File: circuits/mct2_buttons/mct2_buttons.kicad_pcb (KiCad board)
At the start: 2 copper layers, 62.5 x 28 mm, 35 parts, among them J1 Conn_01x08, SW1 B3F-1052, SW10 B3F-1052, SW11 B3F-1052, SW12 B3F-1052, SW13 OS102011MS2QN1C, SW14 OS102011MS2QN1C, SW2 B3F-1052, SW3 B3F-1052, SW4 B3F-1052, SW5 B3F-1052, SW6 B3F-1052, SW7 B3F-1052, SW8 B3F-1052, SW9 B3F-1052, U1 TCA8418

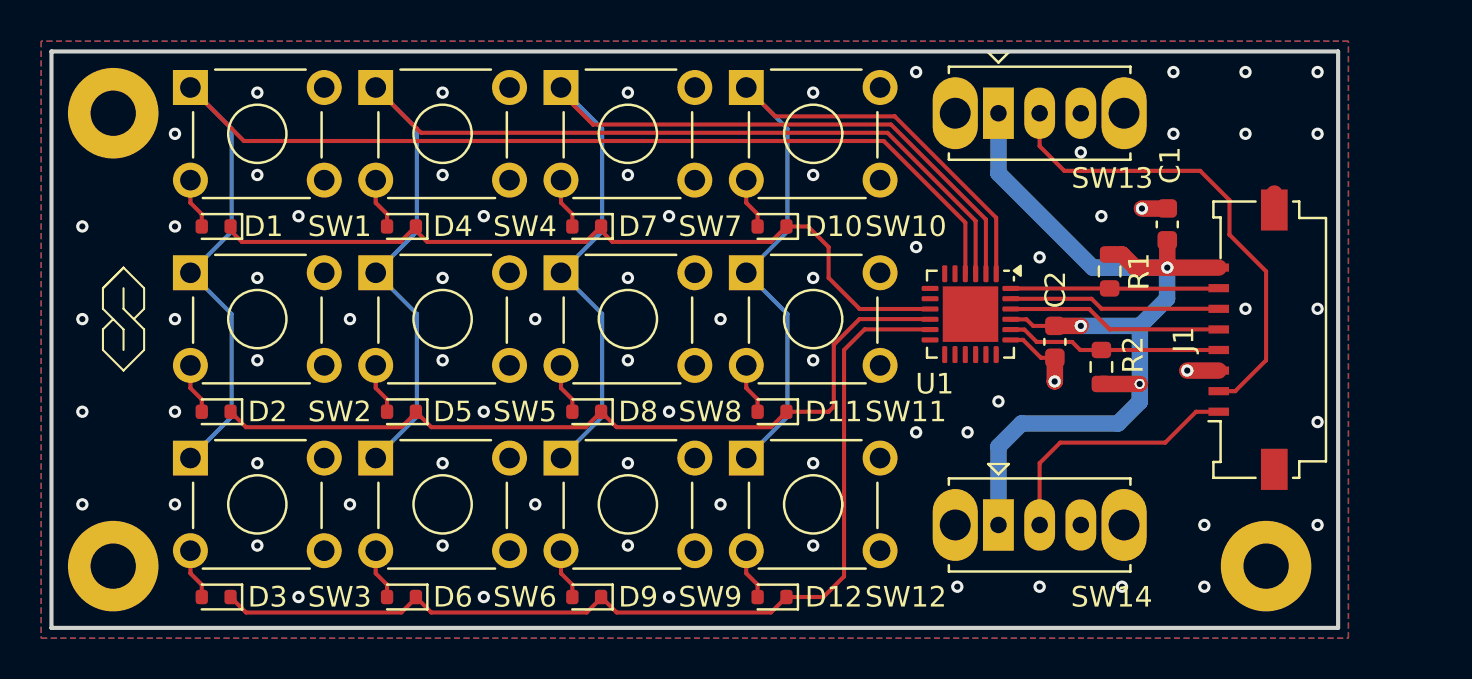
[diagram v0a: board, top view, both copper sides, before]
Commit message: Aug 3, 2024
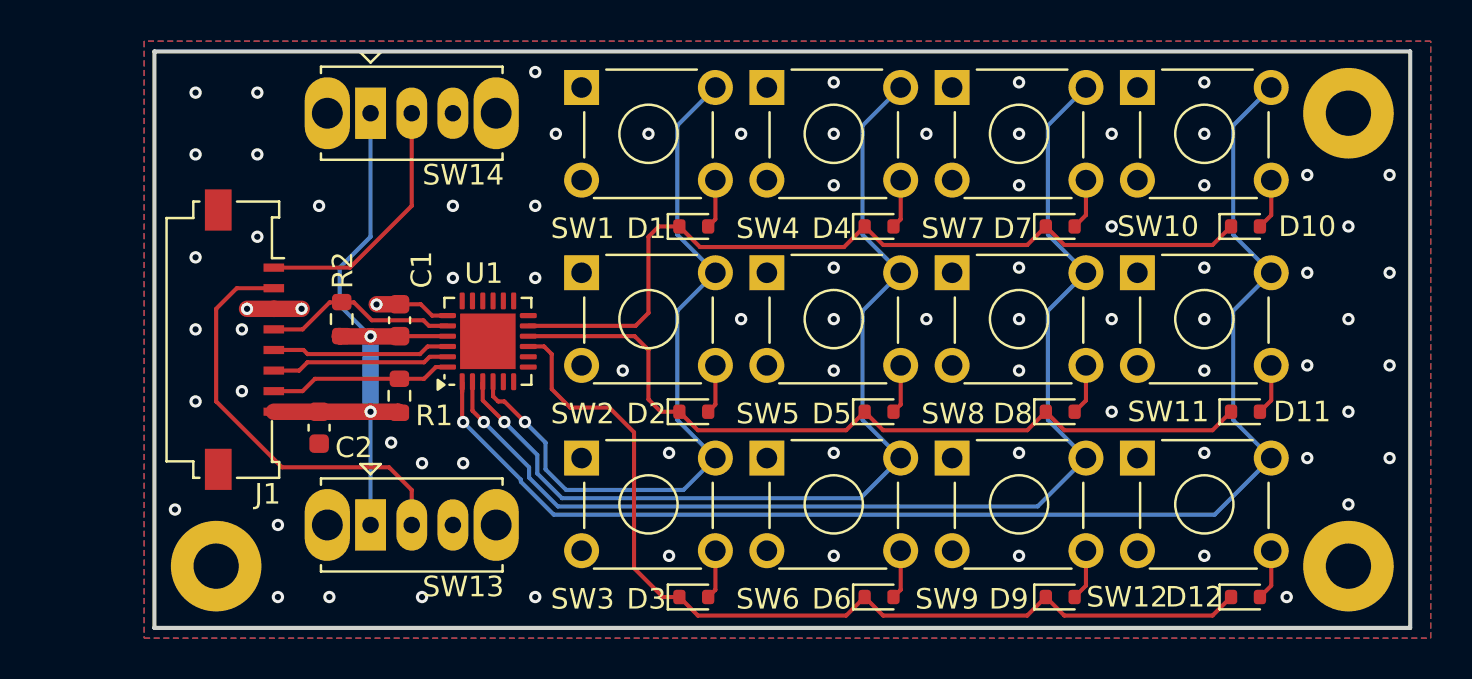
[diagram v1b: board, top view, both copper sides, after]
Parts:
- removed H4: MountingHole, MountingHole:MountingHole_2.2mm_M2_Pad
- added H3: MountingHole, MountingHole:MountingHole_2.2mm_M2_Pad, F.Cu at (98.0, 65.0)
- moved H2 63.9 mm to (98.0, 43.0)
- moved J1 47.7 mm to (44.9, 54.0), turned to -90 degrees
- moved C1 37.6 mm to (51.9, 53.1)
- moved R2 37.0 mm to (49.1, 53.0)
- moved SW13 36.5 mm to (52.5, 63.0)
- moved SW14 36.5 mm to (52.5, 43.0)
- moved C2 36.0 mm to (48.0, 58.3)
- moved R1 35.0 mm to (51.9, 56.7), turned to 90 degrees
- moved U1 23.5 mm to (56.2, 54.1), turned to 90 degrees
- moved D1 23.2 mm to (66.2, 48.5), turned to 0 degrees
- moved D2 23.2 mm to (66.2, 57.5), turned to 0 degrees
- moved D3 23.2 mm to (66.2, 66.5), turned to 0 degrees
- moved D4 23.2 mm to (75.2, 48.5), turned to 0 degrees
- moved D5 23.2 mm to (75.2, 57.5), turned to 0 degrees
- moved D6 23.2 mm to (75.2, 66.5), turned to 0 degrees
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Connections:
- net Net-(D11-K) renamed COL1
- D1 pad 1: Net-(D1-K) -> COL2
- D10 pad 1: Net-(D1-K) -> COL2
- D12 pad 1: Net-(D12-K) -> COL0
- D3 pad 1: Net-(D12-K) -> COL0
- D4 pad 1: Net-(D1-K) -> COL2
- D6 pad 1: Net-(D12-K) -> COL0
- D7 pad 1: Net-(D1-K) -> COL2
- D9 pad 1: Net-(D12-K) -> COL0
- U1 pad 11: Net-(D12-K) -> COL2
- U1 pad 9: Net-(D1-K) -> COL0
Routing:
- net Net-(D12-K): track 47.7 -> 0.00 mm
- net COL0: track 0.00 -> 46.3 mm
- net COL2: track 0.00 -> 40.6 mm
- net Net-(D1-K): track 38.7 -> 0.00 mm
- net Net-(U1-ROW4): track 64.2 -> 35.9 mm, vias 0 -> 1
- net Net-(U1-ROW7): track 38.8 -> 65.9 mm, vias 0 -> 1
- net VCC: track 46.8 -> 32.7 mm, vias 3 -> 2
- net Net-(U1-ROW5): track 55.7 -> 45.6 mm, vias 0 -> 1
- net Net-(U1-ROW6): track 47.4 -> 55.5 mm, vias 0 -> 1
- net Net-(J1-Pin_2): track 23.3 -> 20.7 mm
- net Net-(J1-Pin_5): track 10.5 -> 8.67 mm
- net Net-(J1-Pin_6): track 10.3 -> 8.72 mm
- net Net-(J1-Pin_7): track 10.1 -> 8.92 mm
- net Net-(J1-Pin_4): track 10.6 -> 9.45 mm
- net GND: track 7.21 -> 6.33 mm, vias 71 -> 78
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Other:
- board size 62.5 x 28 mm -> 61 x 28 mm
- board text added: "MediaCow Touch 2 Button Board Rev.B 20240803 CTCL 2021-2024"
- board text removed: "MediaCow Touch 2 Button Board Rev.A 20240801 CTCL 2021-2024"
